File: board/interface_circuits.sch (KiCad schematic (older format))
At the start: 44 parts, among them J1 Conn_01x03, J2 Conn_01x03, Q1 MMBT3904, Q2 MMBT3904, Q3 MMBT3904, Q4 MMBT3904, U1 TPS77633_SO8, U2 STMPS2151_SOT23-5

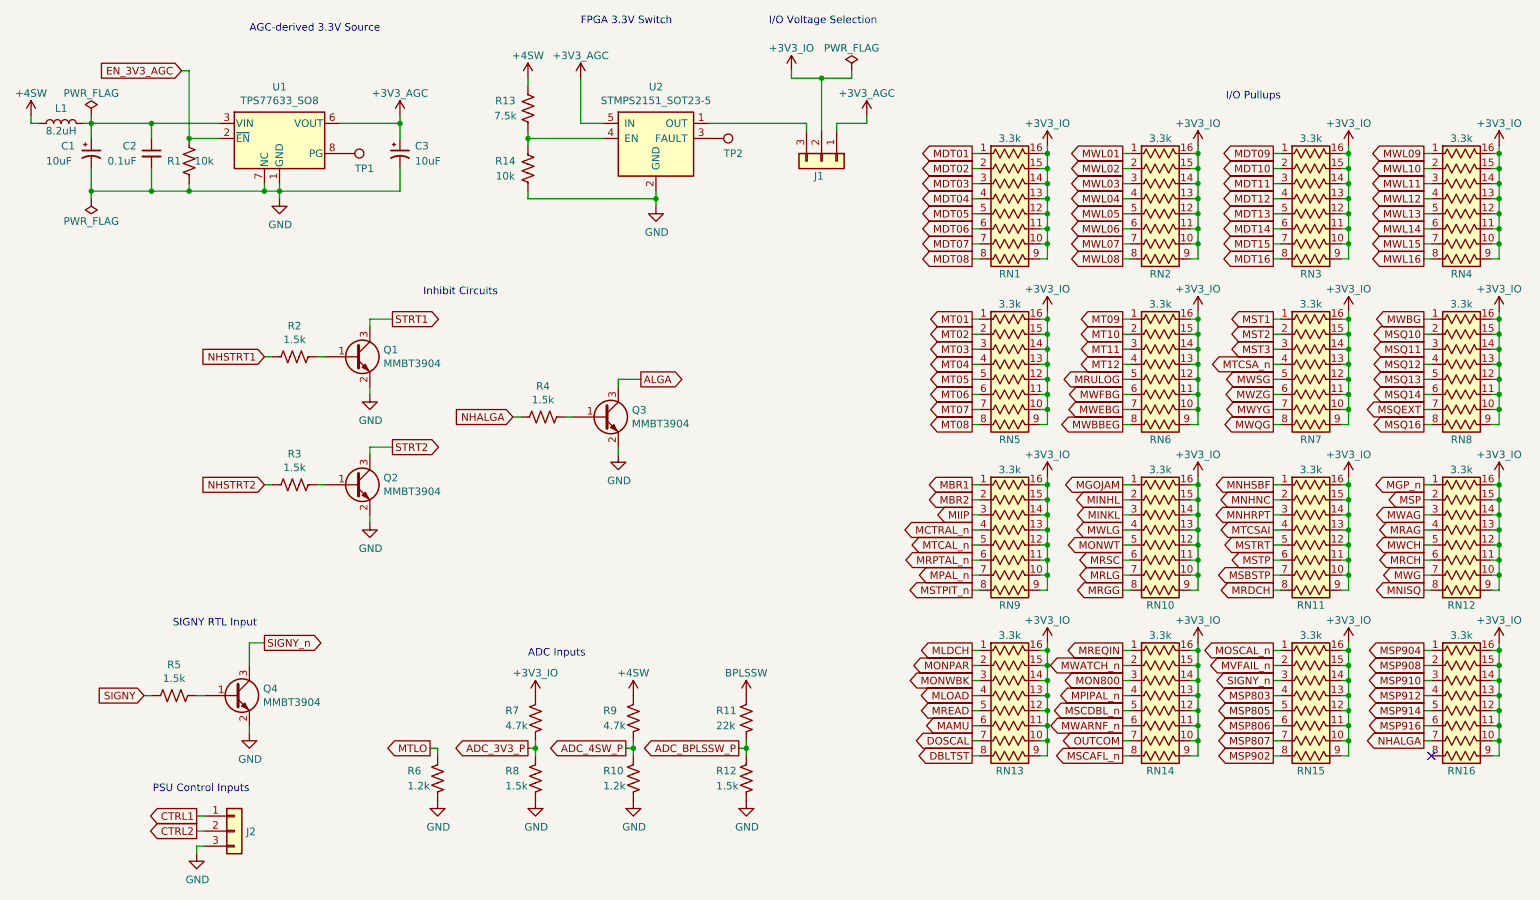
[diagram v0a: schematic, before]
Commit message: Board: more layout work
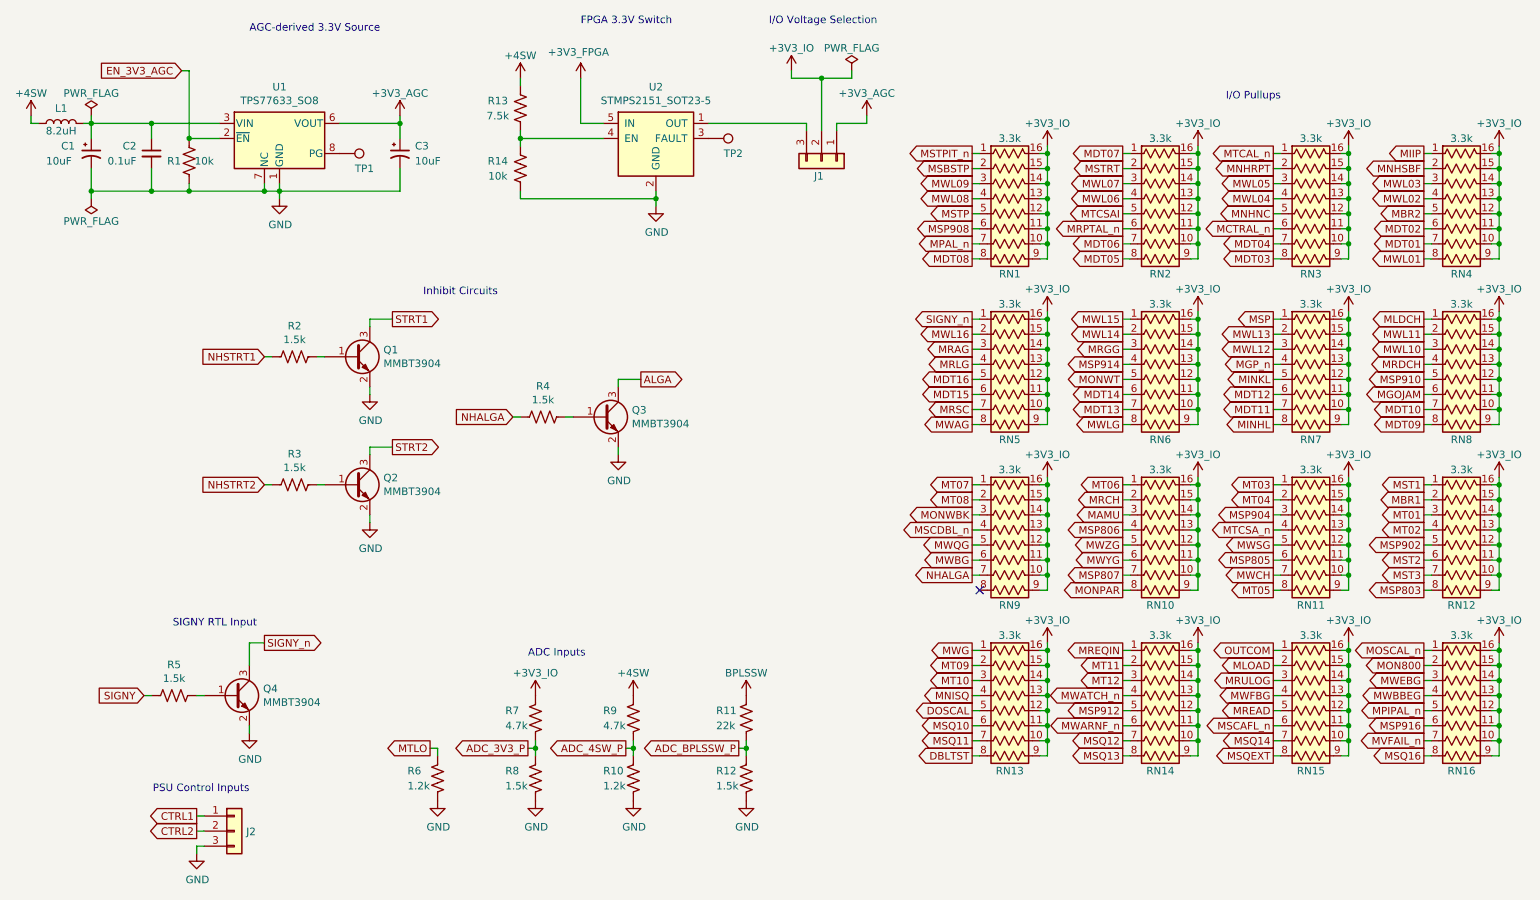
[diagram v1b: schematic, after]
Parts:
- J1: footprint Connector_PinHeader_2.54mm:PinHeader_1x03_P2.54mm_Vertical -> Connector_PinHeader_2.00mm:PinHeader_1x03_P2.00mm_Vertical
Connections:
- net +3V3_AGC: no longer U2.5 (IN)
- net DOSCAL: now also RN13.5 (R5A); no longer RN13.7 (R7A)
- net MAMU: now also RN10.3 (R3A); no longer RN13.6 (R6A)
- net MBR1: now also RN12.2 (R2A); no longer RN9.1 (R1A)
- net MBR2: now also RN4.5 (R5A); no longer RN9.2 (R2A)
- net MCTRAL_n: now also RN3.6 (R6A); no longer RN9.4 (R4A)
- net MDT01: now also RN4.7 (R7A); no longer RN1.1 (R1A)
- net MDT02: now also RN4.6 (R6A); no longer RN1.2 (R2A)
- net MDT03: now also RN3.8 (R8A); no longer RN1.3 (R3A)
- net MDT04: now also RN3.7 (R7A); no longer RN1.4 (R4A)
- net MDT05: now also RN2.8 (R8A); no longer RN1.5 (R5A)
- net MDT06: now also RN2.7 (R7A); no longer RN1.6 (R6A)
- net MDT07: now also RN2.1 (R1A); no longer RN1.7 (R7A)
- net MDT09: now also RN8.8 (R8A); no longer RN3.1 (R1A)
- net MDT10: now also RN8.7 (R7A); no longer RN3.2 (R2A)
- net MDT11: now also RN7.7 (R7A); no longer RN3.3 (R3A)
- net MDT12: now also RN7.6 (R6A); no longer RN3.4 (R4A)
- net MDT13: now also RN6.7 (R7A); no longer RN3.5 (R5A)
- net MDT14: now also RN6.6 (R6A); no longer RN3.6 (R6A)
- net MDT15: now also RN5.6 (R6A); no longer RN3.7 (R7A)
- net MDT16: now also RN5.5 (R5A); no longer RN3.8 (R8A)
- net MGOJAM: now also RN8.6 (R6A); no longer RN10.1 (R1A)
- net MGP_n: now also RN7.4 (R4A); no longer RN12.1 (R1A)
- net MIIP: now also RN4.1 (R1A); no longer RN9.3 (R3A)
- net MINHL: now also RN7.8 (R8A); no longer RN10.2 (R2A)
- net MINKL: now also RN7.5 (R5A); no longer RN10.3 (R3A)
- net MLDCH: now also RN8.1 (R1A); no longer RN13.1 (R1A)
- net MLOAD: now also RN15.2 (R2A); no longer RN13.4 (R4A)
- net MNHNC: now also RN3.5 (R5A); no longer RN11.2 (R2A)
- net MNHRPT: now also RN3.2 (R2A); no longer RN11.3 (R3A)
- net MNHSBF: now also RN4.2 (R2A); no longer RN11.1 (R1A)
- net MNISQ: now also RN13.4 (R4A); no longer RN12.8 (R8A)
- net MON800: now also RN16.2 (R2A); no longer RN14.3 (R3A)
- net MONPAR: now also RN10.8 (R8A); no longer RN13.2 (R2A)
- net MONWBK: now also RN9.3 (R3A); no longer RN13.3 (R3A)
- net MONWT: now also RN6.5 (R5A); no longer RN10.5 (R5A)
- net MOSCAL_n: now also RN16.1 (R1A); no longer RN15.1 (R1A)
- net MPAL_n: now also RN1.7 (R7A); no longer RN9.7 (R7A)
- net MPIPAL_n: now also RN16.5 (R5A); no longer RN14.4 (R4A)
- net MRAG: now also RN5.3 (R3A); no longer RN12.4 (R4A)
- net MRCH: now also RN10.2 (R2A); no longer RN12.6 (R6A)
- net MRDCH: now also RN8.4 (R4A); no longer RN11.8 (R8A)
- net MREAD: now also RN15.5 (R5A); no longer RN13.5 (R5A)
- net MRGG: now also RN6.3 (R3A); no longer RN10.8 (R8A)
- net MRLG: now also RN5.4 (R4A); no longer RN10.7 (R7A)
- net MRPTAL_n: now also RN2.6 (R6A); no longer RN9.6 (R6A)
- net MRSC: now also RN5.7 (R7A); no longer RN10.6 (R6A)
- net MRULOG: now also RN15.3 (R3A); no longer RN6.5 (R5A)
- net MSBSTP: now also RN1.2 (R2A); no longer RN11.7 (R7A)
- net MSCAFL_n: now also RN15.6 (R6A); no longer RN14.8 (R8A)
- net MSCDBL_n: now also RN9.4 (R4A); no longer RN14.5 (R5A)
- net MSP: now also RN7.1 (R1A); no longer RN12.2 (R2A)
- net MSP803: now also RN12.8 (R8A); no longer RN15.4 (R4A)
- net MSP805: now also RN11.6 (R6A); no longer RN15.5 (R5A)
- net MSP806: now also RN10.4 (R4A); no longer RN15.6 (R6A)
- net MSP807: now also RN10.7 (R7A); no longer RN15.7 (R7A)
- net MSP902: now also RN12.5 (R5A); no longer RN15.8 (R8A)
- net MSP904: now also RN11.3 (R3A); no longer RN16.1 (R1A)
- net MSP908: now also RN1.6 (R6A); no longer RN16.2 (R2A)
- net MSP910: now also RN8.5 (R5A); no longer RN16.3 (R3A)
- net MSP912: now also RN14.5 (R5A); no longer RN16.4 (R4A)
- net MSP914: now also RN6.4 (R4A); no longer RN16.5 (R5A)
- net MSQ10: now also RN13.6 (R6A); no longer RN8.2 (R2A)
- net MSQ11: now also RN13.7 (R7A); no longer RN8.3 (R3A)
- net MSQ12: now also RN14.7 (R7A); no longer RN8.4 (R4A)
- net MSQ13: now also RN14.8 (R8A); no longer RN8.5 (R5A)
- net MSQ14: now also RN15.7 (R7A); no longer RN8.6 (R6A)
- net MSQ16: now also RN16.8 (R8A); no longer RN8.8 (R8A)
- net MSQEXT: now also RN15.8 (R8A); no longer RN8.7 (R7A)
- net MST1: now also RN12.1 (R1A); no longer RN7.1 (R1A)
- net MST2: now also RN12.6 (R6A); no longer RN7.2 (R2A)
- net MST3: now also RN12.7 (R7A); no longer RN7.3 (R3A)
- net MSTP: now also RN1.5 (R5A); no longer RN11.6 (R6A)
- net MSTPIT_n: now also RN1.1 (R1A); no longer RN9.8 (R8A)
- net MSTRT: now also RN2.2 (R2A); no longer RN11.5 (R5A)
- net MT01: now also RN12.3 (R3A); no longer RN5.1 (R1A)
- net MT02: now also RN12.4 (R4A); no longer RN5.2 (R2A)
- net MT03: now also RN11.1 (R1A); no longer RN5.3 (R3A)
- net MT04: now also RN11.2 (R2A); no longer RN5.4 (R4A)
- net MT05: now also RN11.8 (R8A); no longer RN5.5 (R5A)
- net MT06: now also RN10.1 (R1A); no longer RN5.6 (R6A)
- net MT07: now also RN9.1 (R1A); no longer RN5.7 (R7A)
- net MT08: now also RN9.2 (R2A); no longer RN5.8 (R8A)
- net MT09: now also RN13.2 (R2A); no longer RN6.1 (R1A)
- net MT10: now also RN13.3 (R3A); no longer RN6.2 (R2A)
- net MT11: now also RN14.2 (R2A); no longer RN6.3 (R3A)
- net MT12: now also RN14.3 (R3A); no longer RN6.4 (R4A)
- net MTCAL_n: now also RN3.1 (R1A); no longer RN9.5 (R5A)
- net MTCSAI: now also RN2.5 (R5A); no longer RN11.4 (R4A)
- net MTCSA_n: now also RN11.4 (R4A); no longer RN7.4 (R4A)
- net MVFAIL_n: now also RN16.7 (R7A); no longer RN15.2 (R2A)
- net MWAG: now also RN5.8 (R8A); no longer RN12.3 (R3A)
- net MWATCH_n: now also RN14.4 (R4A); no longer RN14.2 (R2A)
- net MWBBEG: now also RN16.4 (R4A); no longer RN6.8 (R8A)
- net MWBG: now also RN9.6 (R6A); no longer RN8.1 (R1A)
- net MWCH: now also RN11.7 (R7A); no longer RN12.5 (R5A)
- net MWEBG: now also RN16.3 (R3A); no longer RN6.7 (R7A)
- net MWFBG: now also RN15.4 (R4A); no longer RN6.6 (R6A)
- net MWG: now also RN13.1 (R1A); no longer RN12.7 (R7A)
- net MWL01: now also RN4.8 (R8A); no longer RN2.1 (R1A)
- net MWL02: now also RN4.4 (R4A); no longer RN2.2 (R2A)
- net MWL03: now also RN4.3 (R3A); no longer RN2.3 (R3A)
- net MWL04: now also RN3.4 (R4A); no longer RN2.4 (R4A)
- net MWL05: now also RN3.3 (R3A); no longer RN2.5 (R5A)
- net MWL06: now also RN2.4 (R4A); no longer RN2.6 (R6A)
- net MWL07: now also RN2.3 (R3A); no longer RN2.7 (R7A)
- net MWL08: now also RN1.4 (R4A); no longer RN2.8 (R8A)
- net MWL09: now also RN1.3 (R3A); no longer RN4.1 (R1A)
- net MWL10: now also RN8.3 (R3A); no longer RN4.2 (R2A)
- net MWL11: now also RN8.2 (R2A); no longer RN4.3 (R3A)
- net MWL12: now also RN7.3 (R3A); no longer RN4.4 (R4A)
- net MWL13: now also RN7.2 (R2A); no longer RN4.5 (R5A)
- net MWL14: now also RN6.2 (R2A); no longer RN4.6 (R6A)
- net MWL15: now also RN6.1 (R1A); no longer RN4.7 (R7A)
- net MWL16: now also RN5.2 (R2A); no longer RN4.8 (R8A)
- net MWLG: now also RN6.8 (R8A); no longer RN10.4 (R4A)
- net MWQG: now also RN9.5 (R5A); no longer RN7.8 (R8A)
- net MWSG: now also RN11.5 (R5A); no longer RN7.5 (R5A)
- net MWYG: now also RN10.6 (R6A); no longer RN7.7 (R7A)
- net MWZG: now also RN10.5 (R5A); no longer RN7.6 (R6A)
- net NHALGA: now also RN9.7 (R7A); no longer RN16.7 (R7A)
- net OUTCOM: now also RN15.1 (R1A); no longer RN14.7 (R7A)
- net SIGNY_n: now also RN5.1 (R1A); no longer RN15.3 (R3A)
- new net +3V3_FPGA: U2.5 (IN)
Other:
- moved on the sheet: R13, R14
